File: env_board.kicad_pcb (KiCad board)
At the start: 2 copper layers, 21 x 23 mm, 26 parts, among them J1 CONN_01X07, J2 BATT_CONN, P1 USB_OTG, Q1 Q_NMOS_GSD, Q2 Q_PMOS_GSD, U1 RFD77101, U2 ENS210, U3 CCS811, U4 TLV74130, U5 MCP73811T-420I-OT, U6 BMP280

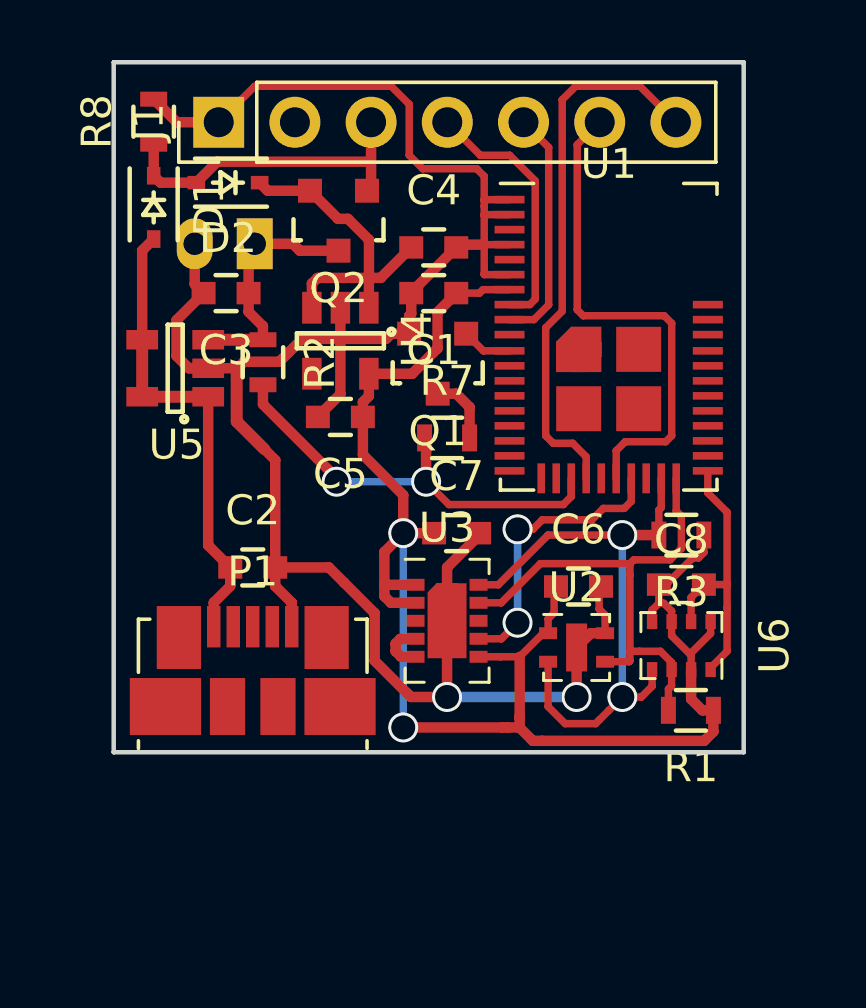
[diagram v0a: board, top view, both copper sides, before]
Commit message: update sensor/housings
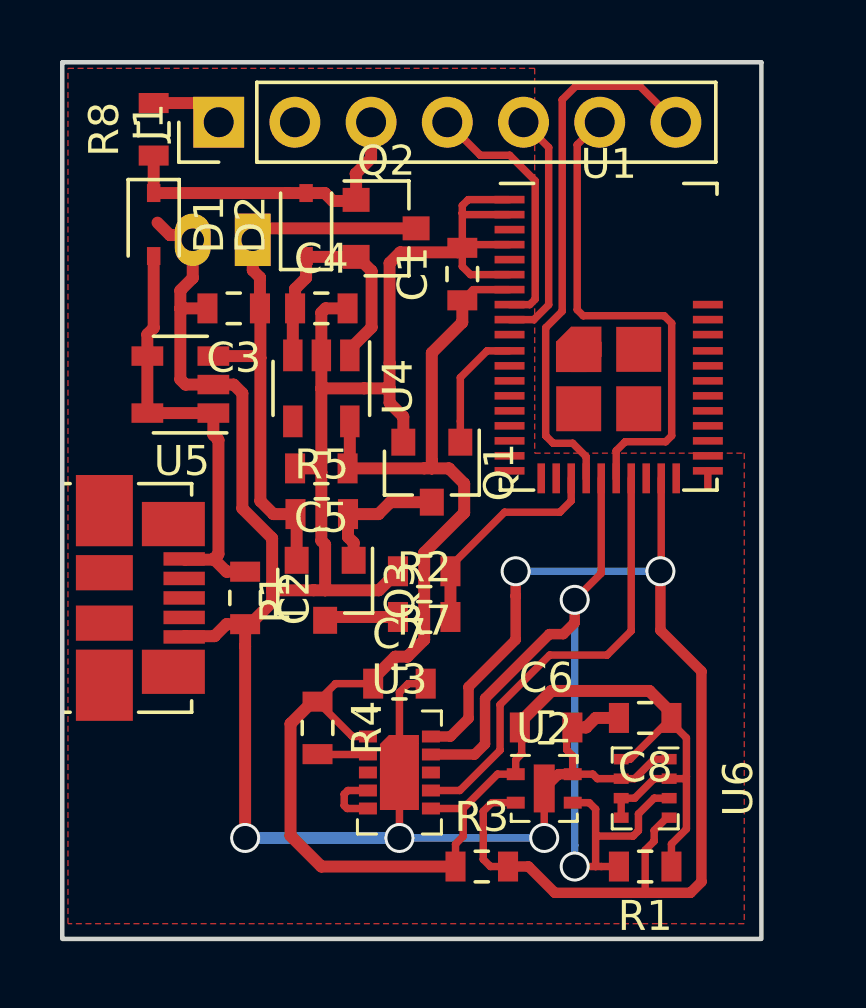
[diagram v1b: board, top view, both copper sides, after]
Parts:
- added Q3: DMP3099L-13, Package_TO_SOT_SMD:SOT-23, F.Cu at (155.0, 114.6)
- added R4: 10k, Resistor_SMD:R_0603_1608Metric, F.Cu at (154.8, 119.2)
- added R5: 10k, Resistor_SMD:R_0603_1608Metric, F.Cu at (154.9, 112.1)
- C1, C2, C3, C4, C5, C6, C7, C8: footprint Capacitors_SMD:C_0603 -> Capacitor_SMD:C_0603_1608Metric
- D1, D2: footprint Diodes_SMD:SOD-323 -> Diode_SMD:D_SOD-323
- J1: footprint Pin_Headers:Pin_Header_Straight_1x07_Pitch2.54mm -> Connector_PinHeader_2.54mm:PinHeader_1x07_P2.54mm_Vertical
- J2: footprint Connectors_JST:JST_PH_S2B-PH-K_02x2.00mm_Angled -> Connector_JST:JST_PH_S2B-PH-K_1x02_P2.00mm_Horizontal
- P1: footprint Connectors_USB:USB_Micro-B_Molex_47346-0001 -> Connector_USB:USB_Micro-B_Molex_47346-0001
- Q1: value Q_NMOS_GSD -> NX7002AKVL; footprint TO_SOT_Packages_SMD:SOT-23 -> Package_TO_SOT_SMD:SOT-23
- Q2: value Q_PMOS_GSD -> DMP3099L-13; footprint TO_SOT_Packages_SMD:SOT-23 -> Package_TO_SOT_SMD:SOT-23
- R1, R2, R3, R7, R8: footprint Resistors_SMD:R_0603 -> Resistor_SMD:R_0603_1608Metric
- U1: footprint kicad-RF_Modules:RFDigital_RFD77101 -> RF_Module:RFDigital_RFD77101
- U2: footprint Housings_DFN_QFN:AMS_QFN-4-1EP_2x2mm_Pitch0.95mm -> Package_DFN_QFN:AMS_QFN-4-1EP_2x2mm_P0.95mm_EP0.7x1.6mm
- U3: footprint kicad-Housings_LGA:AMS_LGA-10-1EP_2.7x4mm_Pitch0.6mm -> Package_LGA:AMS_LGA-10-1EP_2.7x4mm_P0.6mm
- U4, U5: footprint TO_SOT_Packages_SMD:SOT-23-5 -> Package_TO_SOT_SMD:SOT-23-5
- U6: footprint Housings_LGA:Bosch_LGA-8_2x2.5mm_Pitch0.65mm -> Package_LGA:Bosch_LGA-8_2x2.5mm_P0.65mm_ClockwisePinNumbering
- moved R3 12.9 mm to (160.3, 123.8), turned to 0 degrees
- moved R2 10.0 mm to (158.3, 115.5), turned to 0 degrees
- moved R1 5.43 mm to (165.7, 123.8)
- moved C7 5.37 mm to (157.5, 117.7)
- moved U3 5.30 mm to (157.5, 120.7)
- moved P1 5.21 mm to (148.9, 114.9), turned to 270 degrees
- moved U6 4.91 mm to (165.7, 121.2)
- moved C6 4.82 mm to (162.4, 119.2)
- moved U2 4.82 mm to (162.4, 121.2)
- moved C8 4.61 mm to (165.7, 118.9), turned to 180 degrees
- moved R7 4.51 mm to (158.3, 114.0), turned to 180 degrees
- moved C4 4.26 mm to (154.9, 105.2)
- moved Q1 3.62 mm to (158.6, 110.7), turned to 270 degrees
- moved D2 2.95 mm to (154.4, 102.4), turned to 90 degrees
- moved C5 1.83 mm to (154.9, 110.5)
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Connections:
- net /PowerMgmt/BATT_V renamed /BATT_V
- net /PowerMgmt/BATT_V_EN renamed /BATT_V_EN
- R2 pad 1: +BATT -> Net-(Q3-Pad3)
- R7 pad 2: Net-(Q1-Pad3) -> GND
- U1 pad 24: (no net) -> /SDA
- U1 pad 29: /SDA -> (no net)
- U3 pad 2: VDD -> Net-(R4-Pad2)
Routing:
- net /SCL: track 20.3 -> 39.6 mm
- net /SDA: track 17.2 -> 29.1 mm, vias 0 -> 2
- net +BATT: track 8.40 -> 19.1 mm
- net VDD: track 52.5 -> 60.6 mm, vias 2 -> 0
- net GND: track 84.6 -> 92.4 mm, vias 2 -> 3
- net /BATT_V: track 14.6 -> 7.37 mm, vias 2 -> 0
- net /CCS_WAKE: track 9.58 -> 14.9 mm, vias 2 -> 0
- net /BATT_V_EN: track 1.68 -> 4.16 mm
- net Net-(Q3-Pad3): track 0.00 -> 2.47 mm
- net Net-(C4-Pad1): track 11.3 -> 9.00 mm
- net Net-(Q1-Pad3): track 2.27 -> 4.58 mm
- net Net-(R4-Pad2): track 0.00 -> 1.69 mm
- net Net-(C2-Pad1): track 15.9 -> 14.7 mm
- added copper zone on F.Cu, net GND
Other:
- board size 21 x 23 mm -> 23.3 x 29.2 mm
